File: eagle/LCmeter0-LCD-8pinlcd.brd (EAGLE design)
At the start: 55.9 x 50.5 mm, 25 parts, among them IC1 PIC16F876A-X/SP, K2 DS2Y, Q1 20MHz, Q2 BC548, SW1 SPST, SW2 DPDT

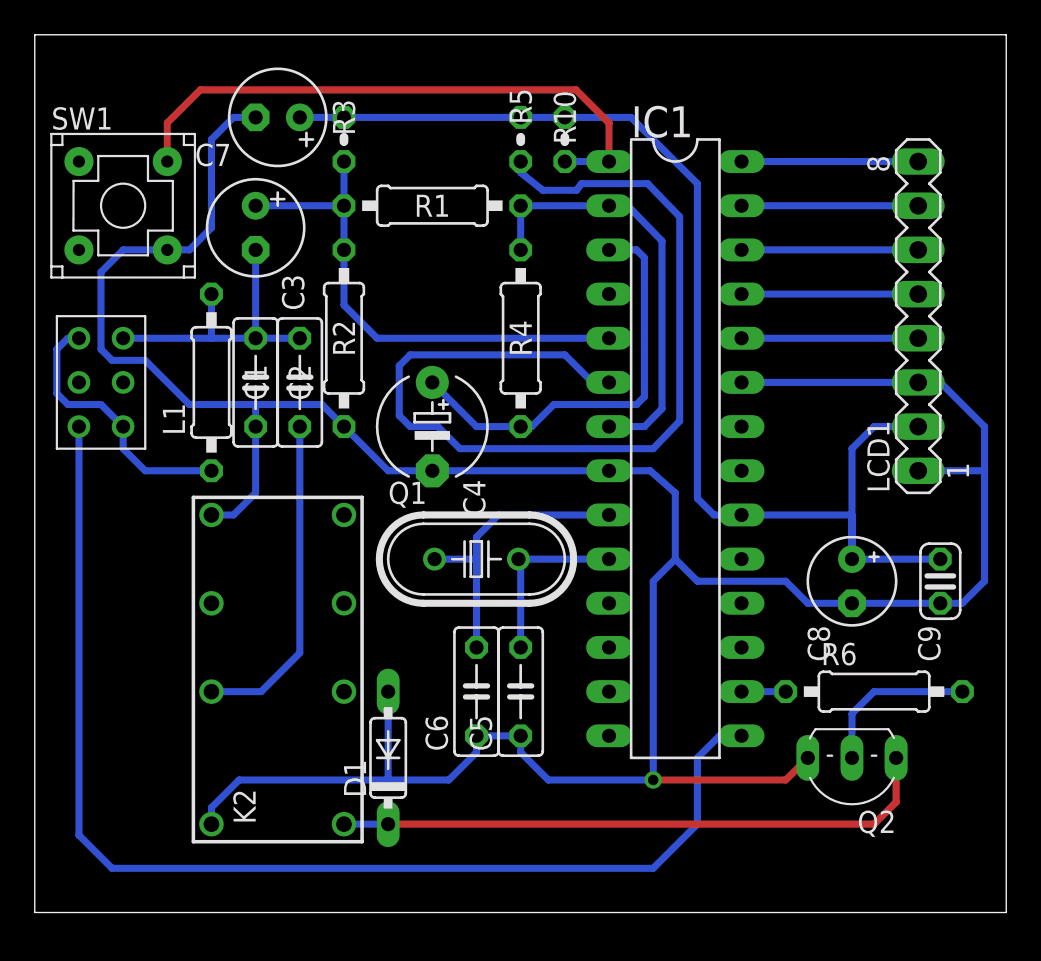
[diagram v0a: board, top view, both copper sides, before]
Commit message: ...
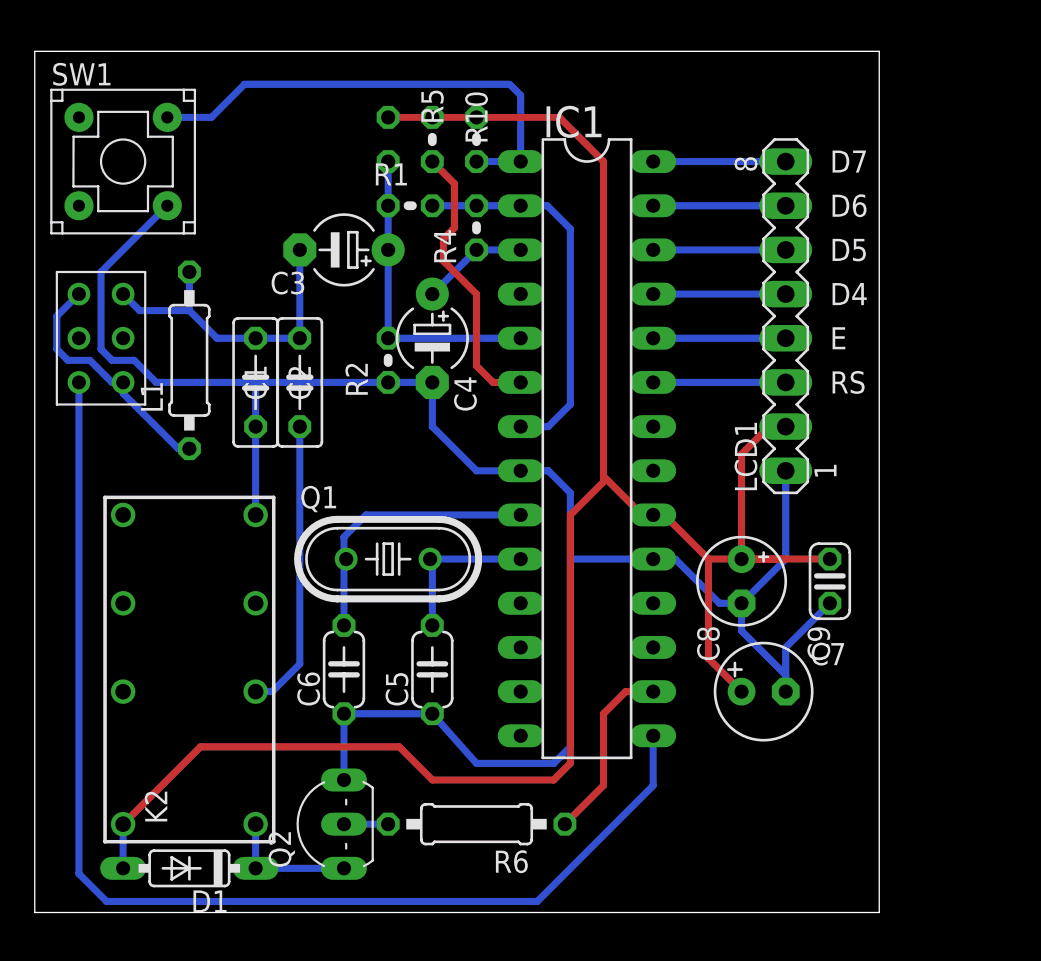
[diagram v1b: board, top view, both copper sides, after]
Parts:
- C3: device rcl:E2,5-6 -> rcl:E5-4
- C4: device rcl:E5-6 -> rcl:E5-4
- C5, C6: device rcl:C050-025X075 -> rcl:C050-024X044
- LCD1: value (none) -> HD44780
- Q1: device crystal:HC49U70 -> crystal:HC49U-V
- R1, R2, R4: device resistor:0207/10 -> resistor:0204V
- R6: value (none) -> 10kΩ
- moved C7 43.3 mm to (41.9, 12.7), turned to 0 degrees
- moved Q2 30.6 mm to (16.5, 5.08), turned to 90 degrees
- moved R6 24.1 mm to (25.4, 5.08), turned to 180 degrees
- moved D1 13.1 mm to (8.89, 2.54), turned to 180 degrees
- moved C6 7.73 mm to (17.8, 14.0)
- moved LCD1 7.62 mm to (43.2, 34.3)
- moved R4 6.84 mm to (25.4, 39.4)
- moved C8 6.35 mm to (40.6, 19.1)
- moved C9 6.35 mm to (45.7, 19.1)
- moved C5 5.24 mm to (22.9, 14.0)
- moved C3 5.24 mm to (17.8, 38.1), turned to 180 degrees
- moved C4 5.08 mm to (22.9, 33.0)
- moved R10 5.08 mm to (25.4, 44.5)
- moved R5 5.08 mm to (22.9, 44.5)
- moved K2 5.08 mm to (8.89, 14.0)
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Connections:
- removed net N$1: C2.2, K2.13
- removed net VSS: C1.2, C4.-, C5.1, C6.1, C7.-, C8.-, C9.2, D1.A, IC1.19, IC1.8, K2.16, K2.9, LCD1.1, Q2.E, R2.1, SW1.1
- new net C2_CON: C2.2, K2.4
- new net GND: C1.2, C4.-, C5.1, C6.1, C7.-, C8.-, C9.2, IC1.19, IC1.8, K2.8, LCD1.1, Q2.E, R2.1, SW1.1
- net VCC: now also D1.A, K2.16
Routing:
- net VSS: track 161.9 -> 0.00 mm, vias 1 -> 0
- net GND: track 0.00 -> 114.3 mm
- net VCC: track 70.1 -> 115.3 mm
- net A4: track 56.3 -> 16.3 mm
- net /RELAY: track 34.8 -> 7.62 mm
- net N$1: track 19.0 -> 0.00 mm
- net A1: track 24.2 -> 6.58 mm
- net C2_CON: track 0.00 -> 16.9 mm
- net A3: track 29.4 -> 17.8 mm
- net RC5: track 2.54 -> 10.7 mm
- net N$5: track 9.42 -> 2.54 mm
- net /MCLR: track 34.0 -> 27.7 mm
- net A0: track 24.6 -> 22.0 mm
- net RS: track 10.2 -> 7.62 mm
- net E: track 10.2 -> 7.62 mm
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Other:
- board size 55.9 x 50.5 mm -> 48.6 x 49.5 mm
- board text added: "D4"
- board text added: "D5"
- board text added: "D6"
- board text added: "D7"
- board text added: "E"
- board text added: "RS"
